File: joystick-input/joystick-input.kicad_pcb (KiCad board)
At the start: 2 copper layers, 53.3 x 38.6 mm, 11 parts, among them J1 Conn_01x18_Male

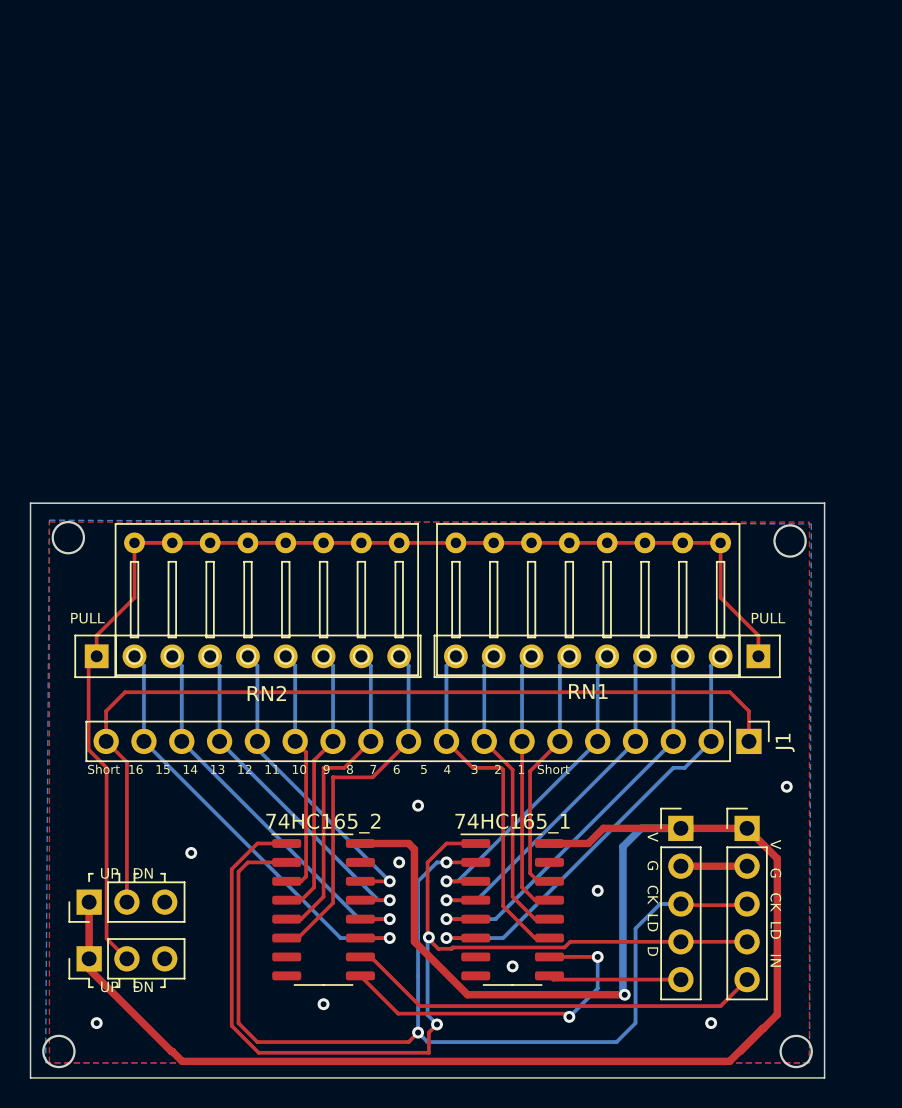
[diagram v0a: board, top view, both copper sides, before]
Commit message: joystick 보드 원복
Signed-off-by: Ju, Gyeong-min <jcmh74@gmail.com>
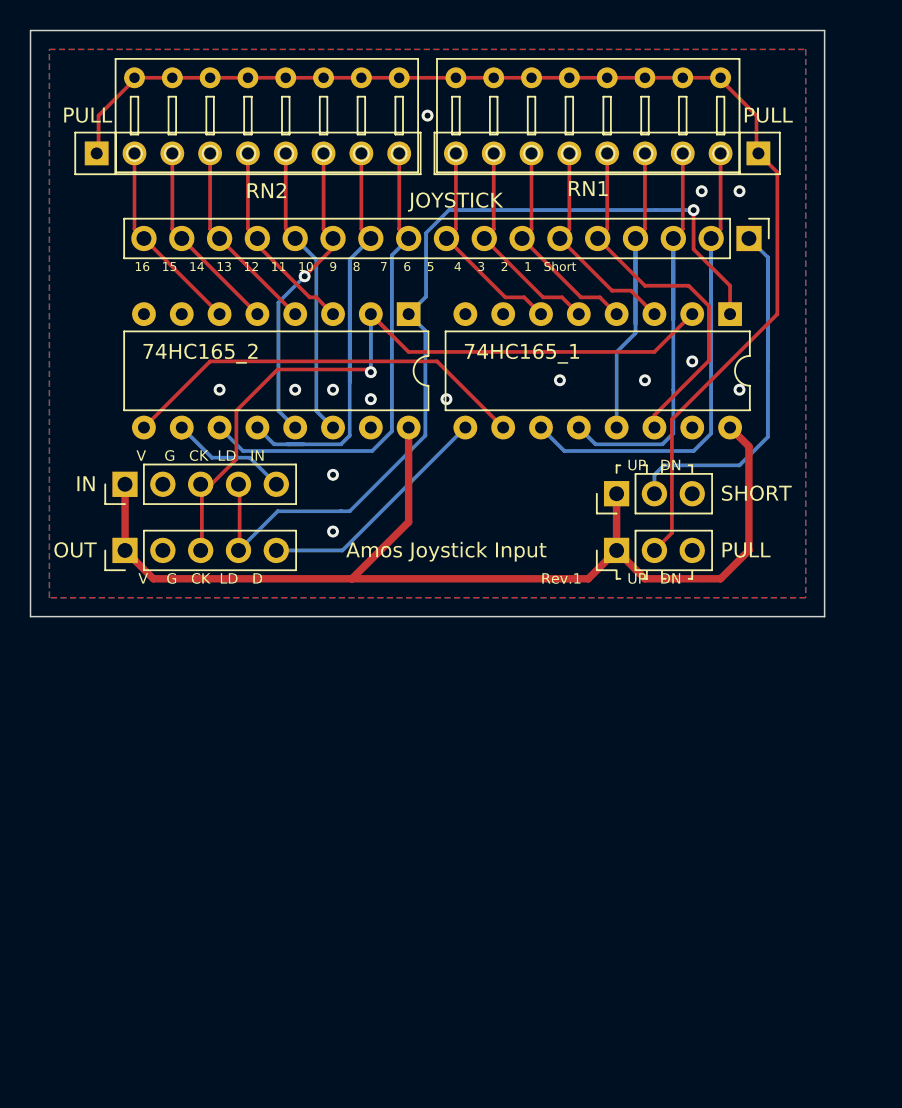
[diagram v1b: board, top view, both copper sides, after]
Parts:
- removed IN1, OUT1: Conn_01x05_Male, Connector_PinHeader_2.54mm:PinHeader_1x05_P2.54mm_Vertical
- removed J1: Conn_01x18_Male, Connector_PinHeader_2.54mm:PinHeader_1x18_P2.54mm_Vertical
- removed PULL1, SHORT1: Conn_01x03_Male, Connector_PinHeader_2.54mm:PinHeader_1x03_P2.54mm_Vertical
- added IN: Conn_01x05_Male, Connector_PinHeader_2.54mm:PinHeader_1x05_P2.54mm_Vertical, F.Cu at (118.1, 61.0)
- added JOYSTICK: Conn_01x17_Male, Connector_PinHeader_2.54mm:PinHeader_1x17_P2.54mm_Vertical, F.Cu at (160.0, 44.5)
- added OUT: Conn_01x05_Male, Connector_PinHeader_2.54mm:PinHeader_1x05_P2.54mm_Vertical, F.Cu at (118.1, 65.4)
- added PULL: Conn_01x03_Male, Connector_PinHeader_2.54mm:PinHeader_1x03_P2.54mm_Vertical, F.Cu at (151.1, 65.4)
- added SHORT: Conn_01x03_Male, Connector_PinHeader_2.54mm:PinHeader_1x03_P2.54mm_Vertical, F.Cu at (151.1, 61.6)
- 74HC165_1, 74HC165_2: footprint Package_SO:SOIC-16_3.9x9.9mm_P1.27mm -> Package_DIP:DIP-16_W7.62mm
- moved 74HC165_1 42.6 mm to (158.8, 49.5), turned to 270 degrees
- moved 74HC165_2 40.4 mm to (137.2, 49.5), turned to 270 degrees
- moved RN1 33.8 mm to (160.7, 38.7)
- moved RN2 33.8 mm to (116.2, 38.7)
- moved H1 31.6 mm to (118.7, 38.7), turned to 90 degrees
- moved H2 31.6 mm to (140.3, 38.7), turned to 90 degrees
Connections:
- 74HC165_1 pad 11: /C_B -> /C_UP
- 74HC165_1 pad 12: /C_A -> /C_DOWN
- 74HC165_1 pad 13: /C_SELECT -> /C_LEFT
- 74HC165_1 pad 14: /C_START -> /C_RIGHT
- 74HC165_1 pad 3: /C_RIGHT -> /C_START
- 74HC165_1 pad 4: /C_LEFT -> /C_SELECT
- 74HC165_1 pad 5: /C_DOWN -> /C_A
- 74HC165_1 pad 6: /C_UP -> /C_B
- 74HC165_2 pad 11: /C_EX4 -> /C_X
- 74HC165_2 pad 12: /C_EX3 -> /C_Y
- 74HC165_2 pad 13: /C_EX2 -> /C_L
- 74HC165_2 pad 14: /C_EX1 -> /C_R
- 74HC165_2 pad 3: /C_R -> /C_EX1
- 74HC165_2 pad 4: /C_L -> /C_EX2
- 74HC165_2 pad 5: /C_Y -> /C_EX3
- 74HC165_2 pad 6: /C_X -> /C_EX4
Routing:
- net VCC: track 123.8 -> 73.8 mm, vias 1 -> 0
- net /C_SHORT: track 59.7 -> 30.8 mm
- net /CLK: track 71.2 -> 50.0 mm, vias 2 -> 1
- net /D_IN: track 28.1 -> 8.64 mm
- net /C_EX4: track 29.9 -> 13.2 mm, vias 1 -> 0
- net /C_Y: track 21.6 -> 36.0 mm
- net /C_EX3: track 26.9 -> 13.2 mm, vias 1 -> 0
- net /C_EX2: track 23.8 -> 13.2 mm, vias 1 -> 0
- net /C_B: track 23.7 -> 14.4 mm
- net /C_EX1: track 21.0 -> 13.4 mm, vias 1 -> 0
- net /C_UP: track 31.2 -> 38.8 mm, vias 1 -> 0
- net /C_X: track 24.6 -> 32.2 mm
- net /LOAD: track 68.3 -> 60.7 mm, vias 2 -> 1
- net /D_OUT: track 8.93 -> 16.1 mm
- net /C_A: track 20.3 -> 14.4 mm
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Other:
- board size 53.3 x 38.6 mm -> 53.3 x 39.4 mm
- board text added: "16 15 14 13 12 11 10 9 8 7 6 5 4 3 2 1 Short"
- board text added: "Rev.1"
- board text removed: "Rev.2"
- board text removed: "Short 16 15 14 13 12 11 10 9 8 7 6 5 4 3 2 1 Short"
